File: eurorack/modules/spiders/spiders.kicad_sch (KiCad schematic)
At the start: 115 parts, among them J1 AudioJack2_SwitchT, J10 Conn_01x08_Female, J11 Conn_02x08_Odd_Even, J12 Conn_02x08_Odd_Even, J2 AudioJack2_SwitchT, J3 AudioJack2_SwitchT, J4 AudioJack2_SwitchT, J5 AudioJack2_SwitchT, J6 AudioJack2_SwitchT, J7 AudioJack2_SwitchT, J8 AudioJack2_SwitchT, J9 Conn_01x08_Male, SW1 SW_Push_LED, SW2 SW_Push_LED, SW3 SW_Push_LED, SW4 SW_Push_LED, SW5 SW_Push_LED, SW6 SW_Push_LED, SW7 SW_Push_LED, SW8 SW_Push_LED, U1 TL074, U10 Chordata, U2 TMUX8212, U3 TL074, U4 TMUX8212, U5 TL074, U6 TMUX8212, U8 TMUX8212

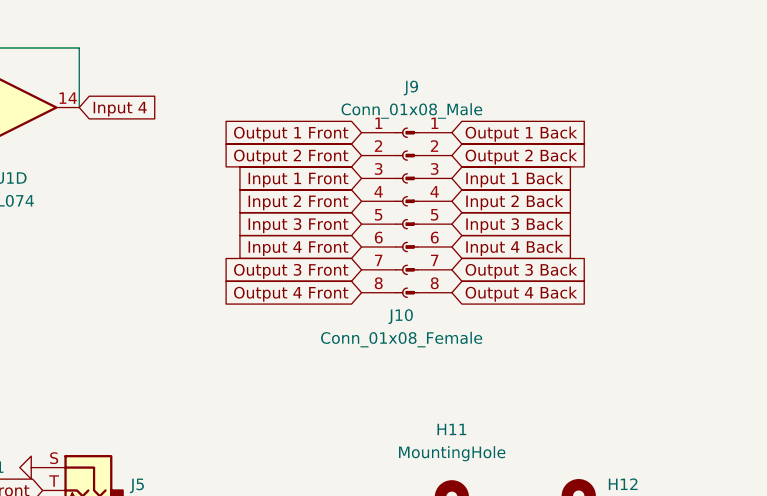
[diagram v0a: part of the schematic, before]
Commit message: spiders tweaks
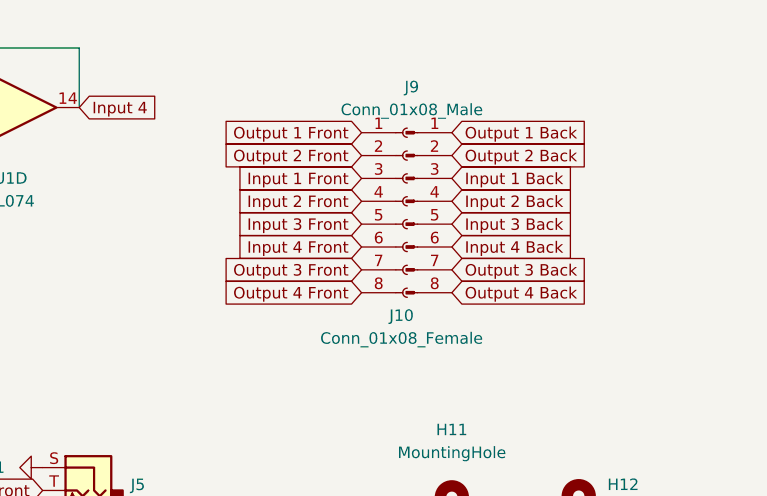
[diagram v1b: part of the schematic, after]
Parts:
- D1, D2, D3, D4, D5, D6, D7, D8: footprint Diode_SMD:D_0805_2012Metric -> Diode_SMD:D_SOD-323_HandSoldering
